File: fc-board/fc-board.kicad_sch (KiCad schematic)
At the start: 9 parts, among them J1 ESQ-125-14-G-D, J2 MSXS-08PFFR-SF7002

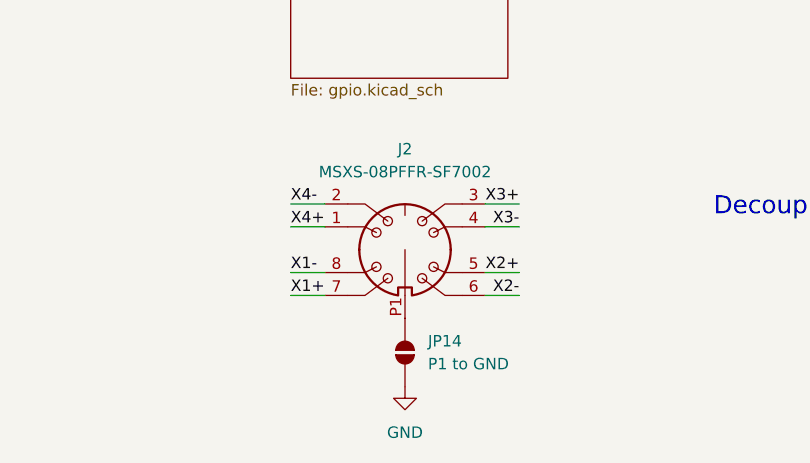
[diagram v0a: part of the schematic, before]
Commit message: Update files to V9
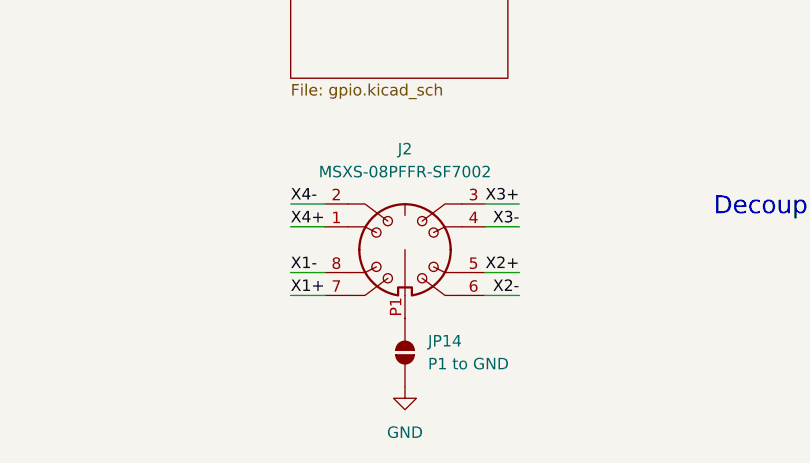
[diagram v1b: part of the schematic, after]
